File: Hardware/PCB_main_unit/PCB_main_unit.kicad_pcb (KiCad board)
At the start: 4 copper layers, 60 x 60 mm, 48 parts, among them J1 Conn_01x03, J10 Conn_01x03, J11 Conn_01x03, J12 Conn_01x04, J13 Conn_01x07, J14 Conn_ST_STDC14, J15 Conn_01x03, J16 Conn_01x02, J2 Conn_01x03, J3 Conn_01x03, J4 Conn_01x03, J5 Conn_01x03, J6 Conn_01x03, J7 Conn_01x03, J8 Conn_01x03, J9 Conn_01x06, SW1 SW_SPDT, U2 STM32G474RETx, U3 AZ1117-3.3

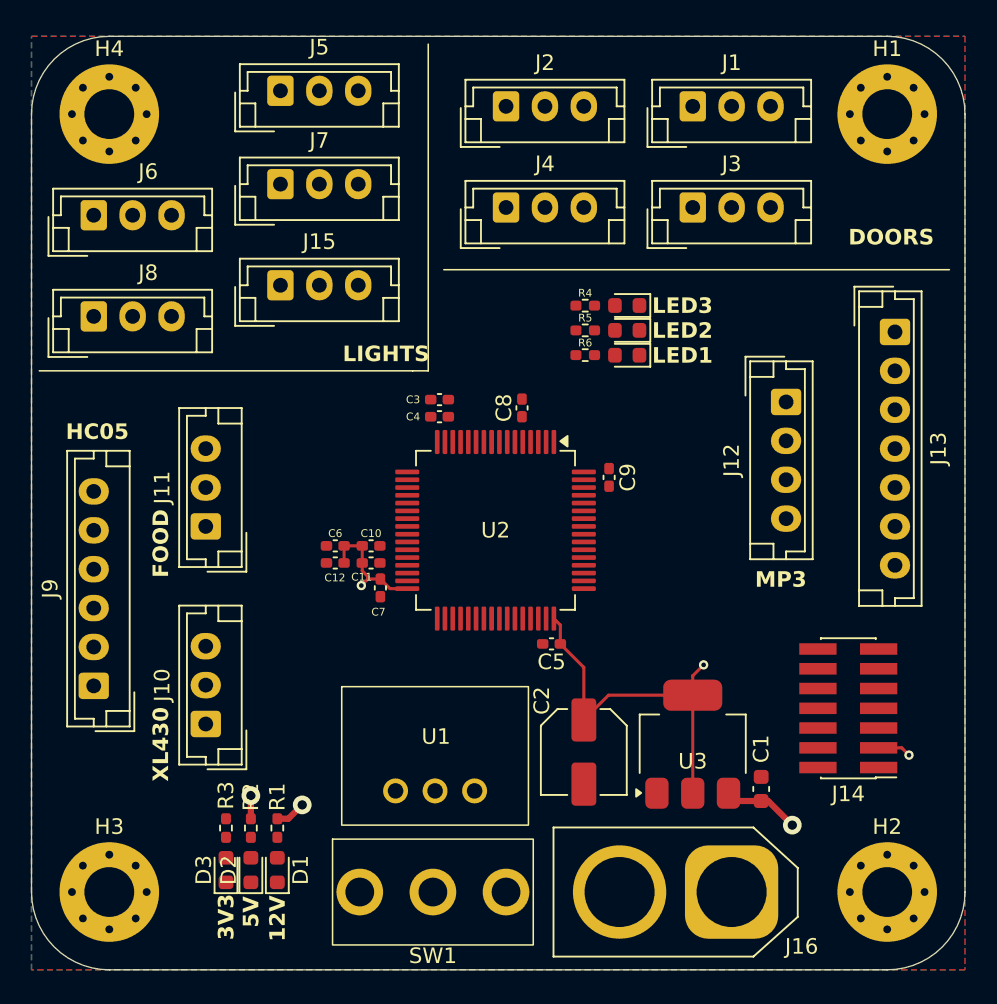
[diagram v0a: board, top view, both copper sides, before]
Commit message: finished main unit PCB
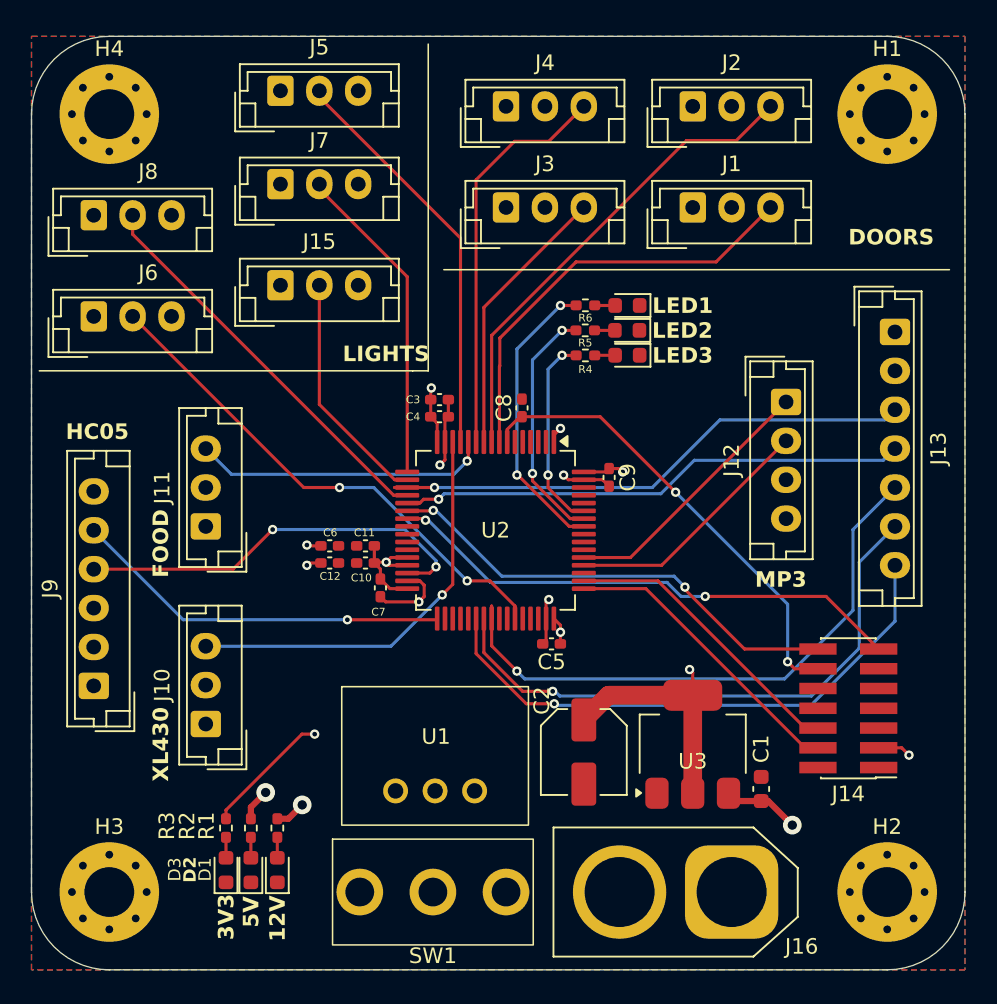
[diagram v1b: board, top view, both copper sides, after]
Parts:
- moved J2 12.0 mm to (160.5, 81.5)
- moved J3 12.0 mm to (148.5, 88.0)
- moved J1 6.50 mm to (160.5, 88.0)
- moved J4 6.50 mm to (148.5, 81.5)
- moved J6 6.50 mm to (122.0, 95.0)
- moved J8 6.50 mm to (122.0, 88.5)
- moved D4 3.20 mm to (156.3, 97.5)
- moved D6 3.20 mm to (156.3, 94.3)
- moved R4 3.20 mm to (153.6, 97.5)
- moved R6 3.20 mm to (153.6, 94.3)
- moved C12 0.36 mm to (137.2, 110.8), turned to 0 degrees
- moved C6 0.36 mm to (137.2, 109.8), turned to 180 degrees
- moved C10 0.36 mm to (139.5, 109.8), turned to 180 degrees
- moved C11 0.36 mm to (139.5, 110.8), turned to 180 degrees
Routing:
- net SPI_CS: track 0.00 -> 38.3 mm, vias 0 -> 1
- net SPI_RST: track 0.00 -> 37.5 mm, vias 0 -> 1
- net SPI_DC: track 0.00 -> 36.4 mm, vias 0 -> 1
- net SPI1_SCK: track 0.00 -> 35.0 mm, vias 0 -> 1
- net UART1_DEBUG_RX: track 0.00 -> 33.8 mm, vias 0 -> 2
- net TIM2_CH3_LIGHT2: track 0.00 -> 33.1 mm, vias 0 -> 2
- net SPI1_MOSI: track 0.00 -> 32.8 mm, vias 0 -> 1
- net TIM1_CH2_DOOR2: track 0.00 -> 30.9 mm
- net UART1_DEBUG_TX: track 0.00 -> 30.2 mm, vias 0 -> 2
- net NRST: track 0.00 -> 30.0 mm, vias 0 -> 2
- net TIM1_CH1_DOOR1: track 0.00 -> 27.6 mm
- net USART2_HD_XL430: track 0.00 -> 26.7 mm, vias 0 -> 1
- net TIM2_CH2_LIGHT1: track 0.00 -> 26.3 mm
- net UART3_TX_HC05: track 0.00 -> 26.3 mm, vias 0 -> 2
- net TIM3_CH1_LIGHT4: track 0.00 -> 25.8 mm
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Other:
- board text added: "D2"
